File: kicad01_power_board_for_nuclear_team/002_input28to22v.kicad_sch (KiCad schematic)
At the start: 0 parts

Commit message: x
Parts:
- added R201: R1206_0.0, 02_dyn_pcblib:R1206mix0603, symbol 01dyn_lib:R1206_0.0
- added R224: R0603_1M, Resistor_SMD:R_0603_1608Metric, symbol 01dyn_lib:R0603_1M
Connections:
- new net V24in: R201.1, R224.2
- new net V24out: R201.2
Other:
- note added: "Note : the input range is 23v to 28v. Please label it on the shell of this power."
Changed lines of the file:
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@@
 (kicad_sch (version 20211123) (generator eeschema)
   (paper "USLetter")
+  (junction (at 64.77 63.5) (diameter 0) (color 0 0 0 0)
+  )
+  (wire (pts (xy 44.45 63.5) (xy 44.45 68.58))
+    (stroke (width 0) (type default) (color 0 0 0 0))
+  )
+  (wire (pts (xy 64.77 63.5) (xy 44.45 63.5))
+    (stroke (width 0) (type default) (color 0 0 0 0))
+  )
+  (wire (pts (xy 113.03 69.85) (xy 64.77 69.85))
+    (stroke (width 0) (type default) (color 0 0 0 0))
+  )
+  (wire (pts (xy 44.45 85.09) (xy 78.74 85.09))
+    (stroke (width 0) (type default) (color 0 0 0 0))
+  )
+  (wire (pts (xy 120.65 69.85) (xy 134.62 69.85))
+    (stroke (width 0) (type default) (color 0 0 0 0))
+  )
+  (wire (pts (xy 44.45 76.2) (xy 44.45 85.09))
+    (stroke (width 0) (type default) (color 0 0 0 0))
+  )
+  (wire (pts (xy 64.77 69.85) (xy 64.77 63.5))
+    (stroke (width 0) (type default) (color 0 0 0 0))
+  )
+  (wire (pts (xy 77.47 63.5) (xy 64.77 63.5))
+    (stroke (width 0) (type default) (color 0 0 0 0))
+  )
+  (text "Note : the input range is 23v to 28v.\nPlease label it on the shell of this power."
+    (at 34.29 40.64 0)
+    (effects (font (size 4 4)) (justify left bottom))
+  )
+  (global_label "V24in" (shape input) (at 77.47 63.5 0) (fields_autoplaced)
+    (effects (font (size 1.27 1.27)) (justify left))
+    (property "Intersheet References" "${INTERSHEET_REFS}" (id 0) (at 85.1445 63.5794 0)
+      (effects (font (size 1.27 1.27)) (justify left) hide)
+    )
+  )
+  (global_label "V24out" (shape input) (at 134.62 69.85 0) (fields_autoplaced)
+    (effects (font (size 1.27 1.27)) (justify left))
+    (property "Intersheet References" "${INTERSHEET_REFS}" (id 0) (at 143.5645 69.7706 0)
+      (effects (font (size 1.27 1.27)) (justify left) hide)
+    )
+  )
+  (symbol (lib_id "01dyn_lib:GND_1") (at 78.74 85.09 0) (unit 1)
+    (in_bom yes) (on_board yes) (fields_autoplaced)
+    (property "Reference" "#PWR0113" (id 0) (at 78.74 91.44 0)
+      (effects (font (size 1.27 1.27)) hide)
+    )
+    (property "Value" "GND_1" (id 1) (at 78.74 88.9 0))
+    (property "Footprint" "" (id 2) (at 78.74 85.09 0)
+      (effects (font (size 1.27 1.27)) hide)
+    )
+    (property "Datasheet" "" (id 3) (at 78.74 85.09 0)
+      (effects (font (size 1.27 1.27)) hide)
+    )
+    (pin "1")
+  )
+  (symbol (lib_id "01dyn_lib:R1206_0.0") (at 116.84 69.85 0) (unit 1)
+    (in_bom yes) (on_board yes) (fields_autoplaced)
+    (property "Reference" "R201" (id 0) (at 116.84 64.77 0)
+      (effects (font (size 1.5 1.5)))
+    )
+    (property "Value" "R1206_0.0" (id 1) (at 115.062 71.247 0)
+      (effects (font (size 0.5 0.5)))
+    )
+    (property "Footprint" "02_dyn_pcblib:R1206mix0603" (id 2) (at 116.84 58.42 0)
+      (effects (font (size 1.27 1.27)) hide)
+    )
+    (property "Datasheet" "~" (id 3) (at 116.84 69.85 90)
+      (effects (font (size 1.27 1.27)) hide)
+    )
+    (property "PartNum" "RC1206FR-070RL" (id 4) (at 116.713 67.945 0)
+      (effects (font (size 1.27 1.27)) hide)
+    )
+    (property "PartDesc" "0 Ohms Jumper 0.25W, 1/4W Chip Resistor 1206 (3216 Metric) Moisture Resistant Thick Film" (id 5) (at 114.3 60.96 0)
+      (effects (font (size 1.27 1.27)) hide)
+    )
+    (pin "1")
+    (pin "2")
+  )
+  (symbol (lib_id "01dyn_lib:R0603_1M") (at 44.45 72.39 90) (unit 1)
+    (in_bom yes) (on_board yes) (fields_autoplaced)
+    (property "Reference" "R224" (id 0) (at 46.99 71.755 90)
+      (effects (font (size 1.5 1.5)) (justify right))
+    )
+    (property "Value" "R0603_1M" (id 1) (at 45.847 74.168 0)
+      (effects (font (size 0.5 0.5)))
+    )
+    (property "Footprint" "Resistor_SMD:R_0603_1608Metric" (id 2) (at 34.29 71.12 0)
+      (effects (font (size 1.27 1.27)) hide)
+    )
+    (property "Datasheet" "~" (id 3) (at 44.45 72.39 90)
+      (effects (font (size 1.27 1.27)) hide)
+    )
+    (property "PartNum" "ERJ-U03F1004V" (id 4) (at 36.83 73.66 0)
+      (effects (font (size 1.27 1.27)) hide)
+    )
+    (property "PartDesc" "1 MOhms ±1% 0.1W, 1/10W Chip Resistor 0603 (1608 Metric) Anti-Sulfur, Automotive AEC-Q200 Thick Film" (id 5) (at 30.48 73.66 0)
+      (effects (font (size 1.27 1.27)) hide)
+    )
+    (pin "1")
+    (pin "2")
+  )
 )

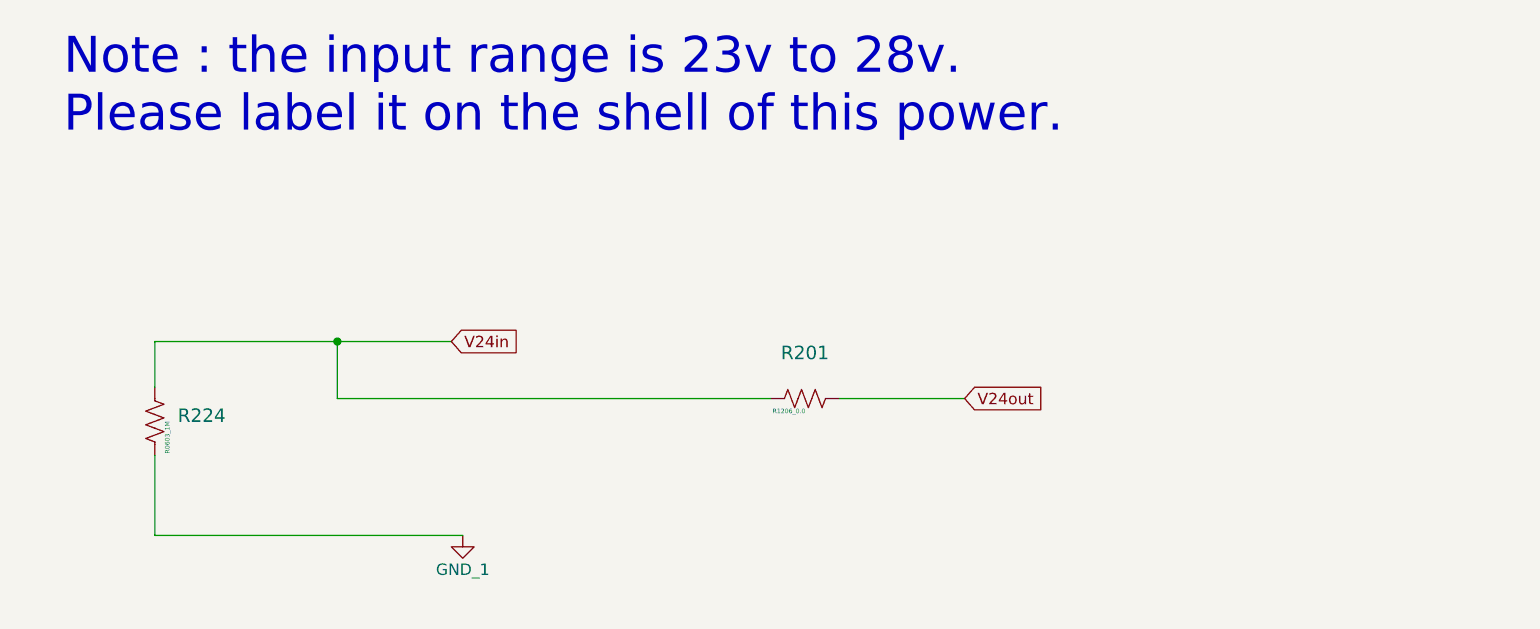
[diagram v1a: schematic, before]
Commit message: ix
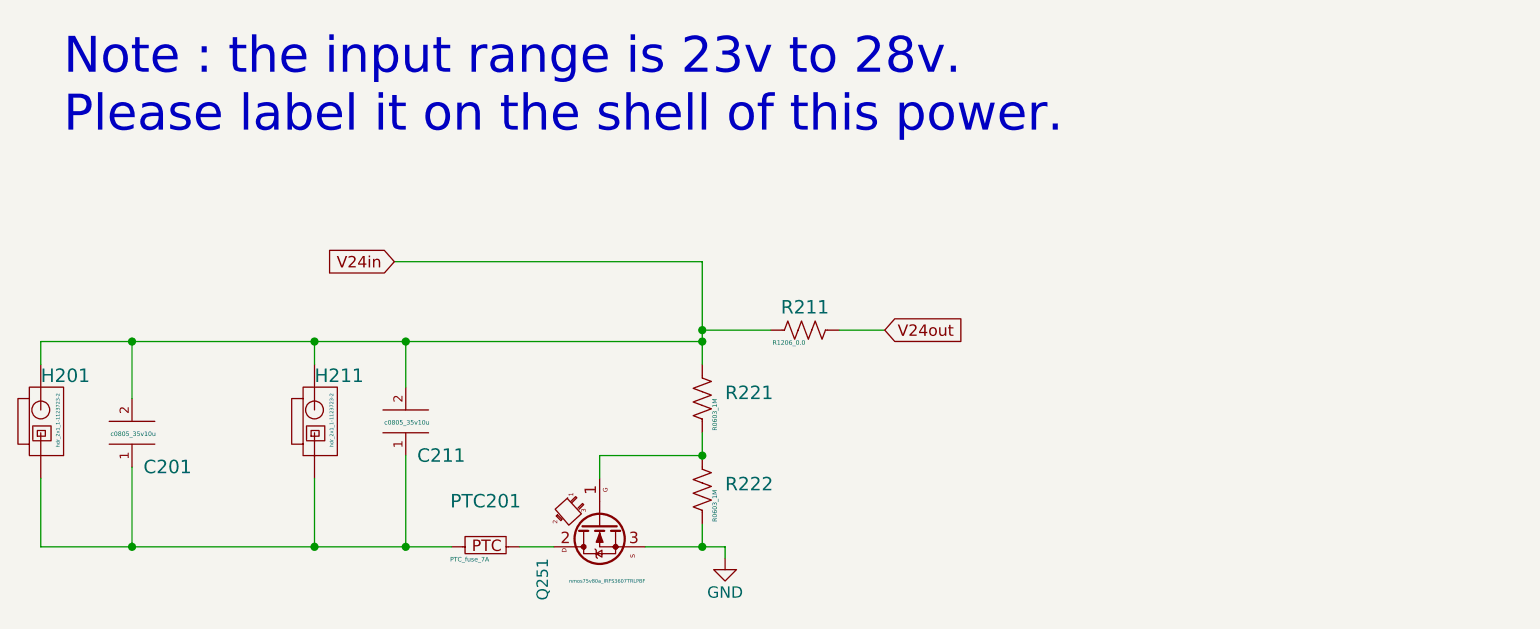
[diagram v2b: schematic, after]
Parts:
- removed R201: R1206_0.0, 02_dyn_pcblib:R1206mix0603, symbol 01dyn_lib:R1206_0.0
- removed R224: R0603_1M, Resistor_SMD:R_0603_1608Metric, symbol 01dyn_lib:R0603_1M
- added C201, C211: c0805_35v10u, 02_dyn_pcblib:C0805mix0603, symbol 1001_un:c0805_35v10u
- added H201, H211: hdr_2x1_1-1123723-2, 02_dyn_pcblib:hdr_2x1_1-1123723-2, symbol 1001_un:hdr_2x1_1-1123723-2
- added PTC201: PTC_fuse_7A, 02_dyn_pcblib:ptc_fuse_2920, symbol 1001_un:PTC_fuse_7A
- added Q251: nmos75v80a_IRFS3607TRLPBF, 02_dyn_pcblib:d2pak_TO263, symbol 1001_un:nmos75v80a_IRFS3607TRLPBF
- added R211: R1206_0.0, 02_dyn_pcblib:R1206mix0603, symbol 1001_un:R1206_0.0
- added R221, R222: R0603_1M, 02_dyn_pcblib:C0603, symbol 1001_un:R0603_1M
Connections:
- net V24in: now also C201.2, C211.2, H201.2, H211.2, R211.1, R221.2
- net V24out: now also R211.2
- new net: Q251.1 (G), R221.1, R222.2
- new net: C201.1, C211.1, H201.1, H211.1, PTC201.1
- new net: PTC201.2, Q251.2 (D)
- new net GND: Q251.3 (S), R222.1
